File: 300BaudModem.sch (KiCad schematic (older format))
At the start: 54 parts

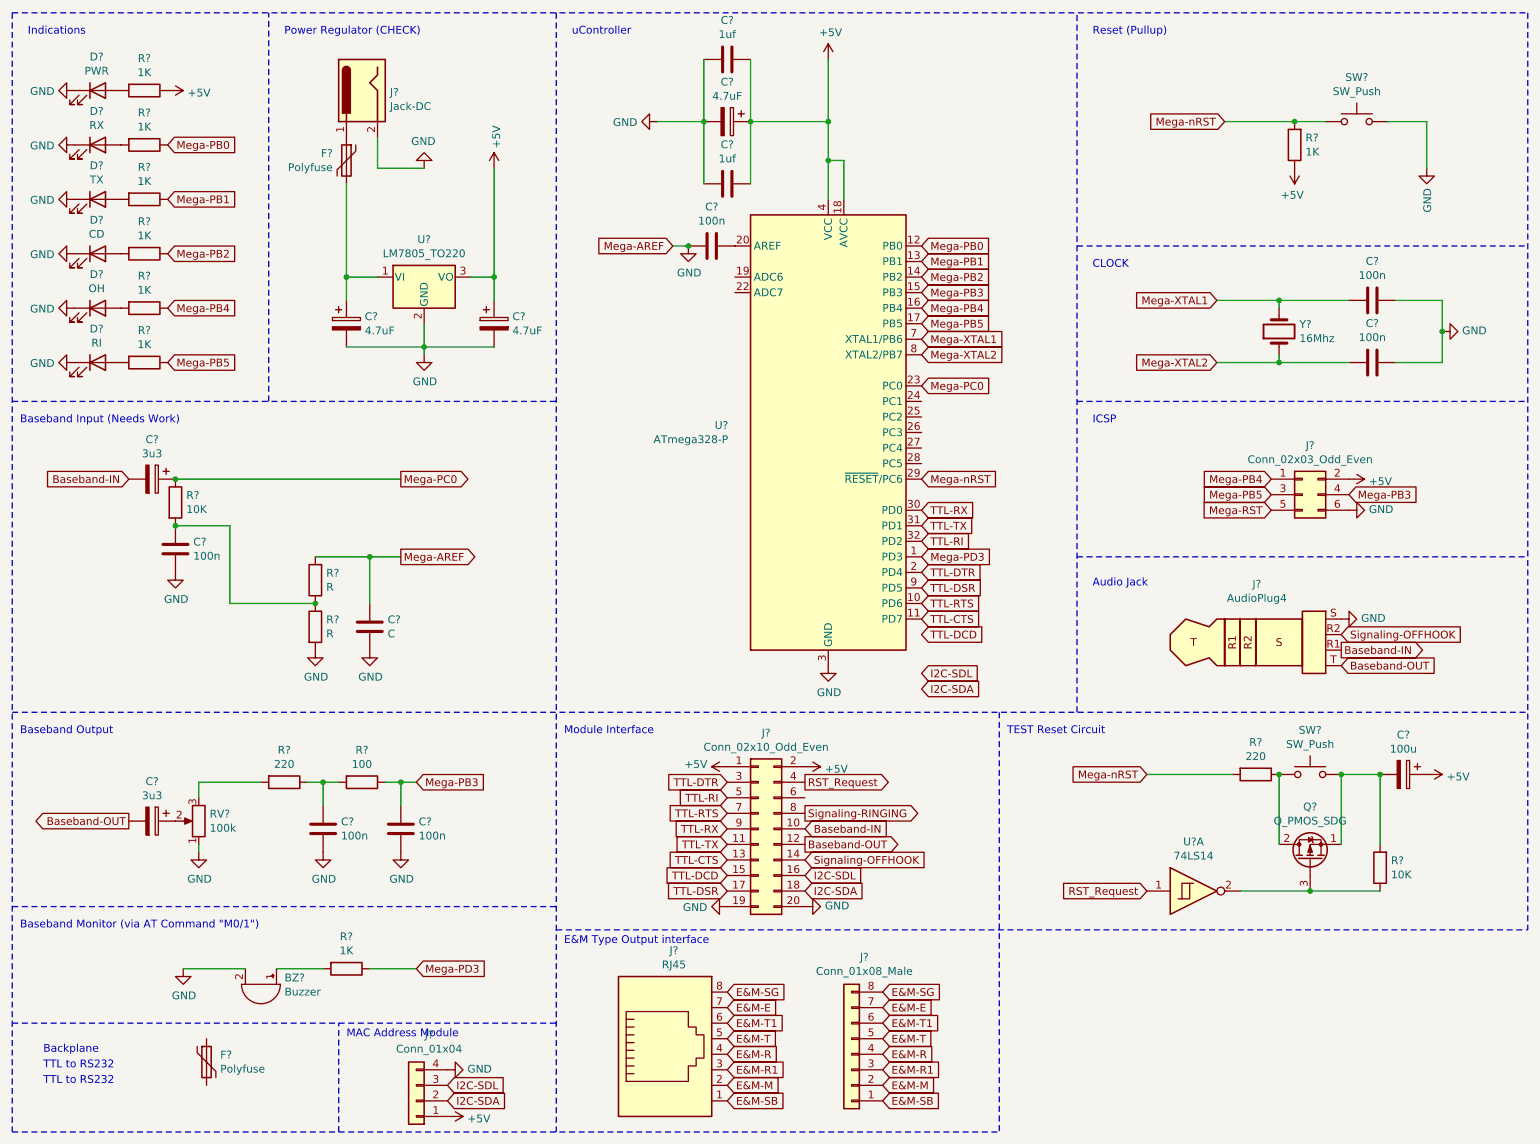
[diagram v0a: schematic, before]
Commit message: updates
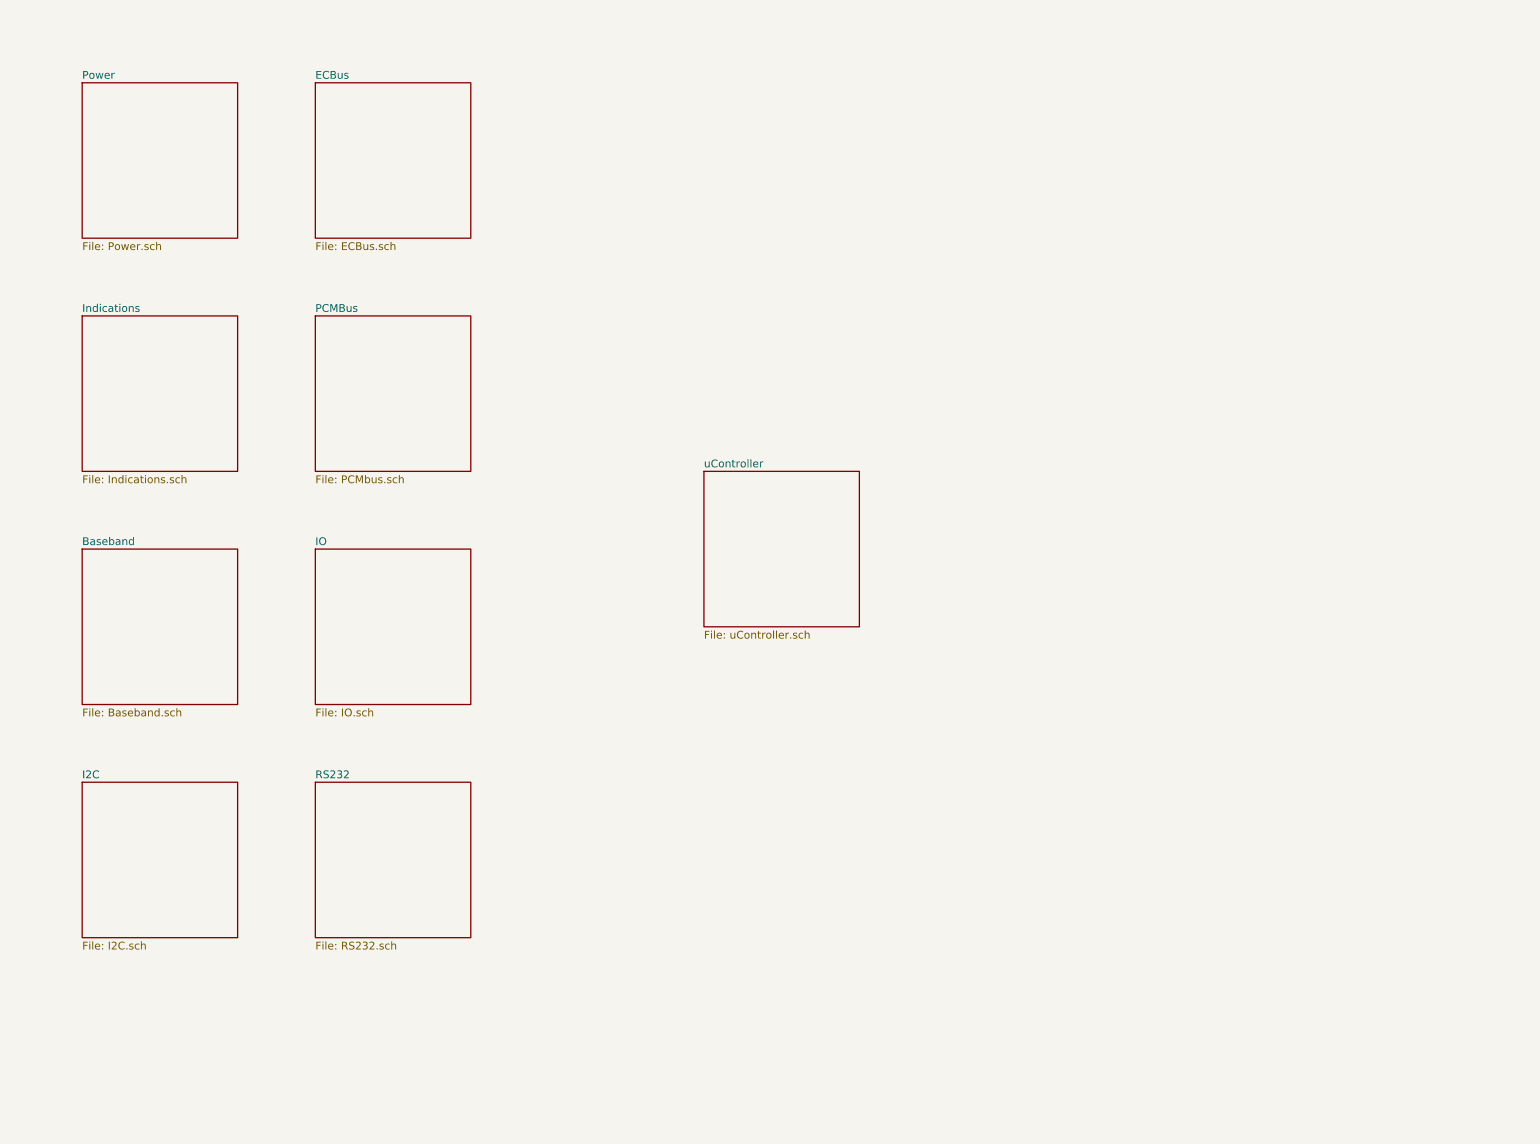
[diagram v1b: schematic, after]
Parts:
- removed BZ?: Buzzer, symbol Device:Buzzer
- removed C? (x2): 3u3, symbol Device:C_Polarized
- removed C? (x6): 100n, symbol Device:C
- removed C?: C, symbol Device:C
- removed C? (x3): 4.7uF, symbol Device:C_Polarized
- removed C? (x2): 1uf, symbol Device:C
- removed C?: 100u, symbol Device:C_Polarized
- removed D?: RX, symbol Device:LED
- removed D?: TX, symbol Device:LED
- removed D?: CD, symbol Device:LED
- removed D?: OH, symbol Device:LED
- removed D?: RI, symbol Device:LED
- removed D?: PWR, symbol Device:LED
- removed F? (x2): Polyfuse, symbol Device:Polyfuse
- removed J?: Conn_02x03_Odd_Even, symbol Connector_Generic:Conn_02x03_Odd_Even
- removed J?: Conn_01x08_Male, symbol Connector_Generic:Conn_01x08
- removed J?: Conn_02x10_Odd_Even, symbol Connector_Generic:Conn_02x10_Odd_Even
- removed J?: RJ45, symbol Connector:RJ45
- removed J?: AudioPlug4, symbol Connector:AudioPlug4
- removed J?: Jack-DC, symbol Connector:Jack-DC
- removed J?: Conn_01x04, symbol Connector_Generic:Conn_01x04
- removed Q?: Q_PMOS_SDG, symbol Device:Q_PMOS_SDG
- removed R? (x2): 10K, symbol Device:R
- removed R? (x2): R, symbol Device:R
- removed R? (x8): 1K, symbol Device:R
- removed R?: 100, symbol Device:R
- removed R? (x2): 220, symbol Device:R
- removed RV?: 100k, symbol Device:R_Potentiometer
- removed SW? (x2): SW_Push, symbol Switch:SW_Push
- removed U?: ATmega328-P, Package_DIP:DIP-28_W7.62mm, symbol MCU_Microchip_ATmega:ATmega328P-A
- removed U?: 74LS14, symbol 74xx:74LS14
- removed U?: LM7805_TO220, Package_TO_SOT_THT:TO-220-3_Vertical, symbol Regulator_Linear:LM7805_TO220
- removed Y?: 16Mhz, symbol Device:Crystal
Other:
- note removed: "Audio Jack"
- note removed: "Backplane"
- note removed: "Baseband Input (Needs Work)"
- note removed: "Baseband Monitor (via AT Command "M0/1")"
- note removed: "Baseband Output"
- note removed: "CLOCK"
- note removed: "E&M Type Output interface"
- note removed: "ICSP"
- note removed: "Indications"
- note removed: "MAC Address Module"
- note removed: "Module Interface"
- note removed: "Power Regulator (CHECK)"
- note removed: "Reset (Pullup)"
- note removed: "TEST Reset Circuit"
- note removed: "TTL to RS232"
- note removed: "uController"
